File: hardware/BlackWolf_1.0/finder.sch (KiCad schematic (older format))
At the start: 13 parts, among them U4 TCA9545A, U5 VL6180X_POLOLU, U6 VL6180X_POLOLU, U7 VL6180X_POLOLU, U8 VL6180X_POLOLU

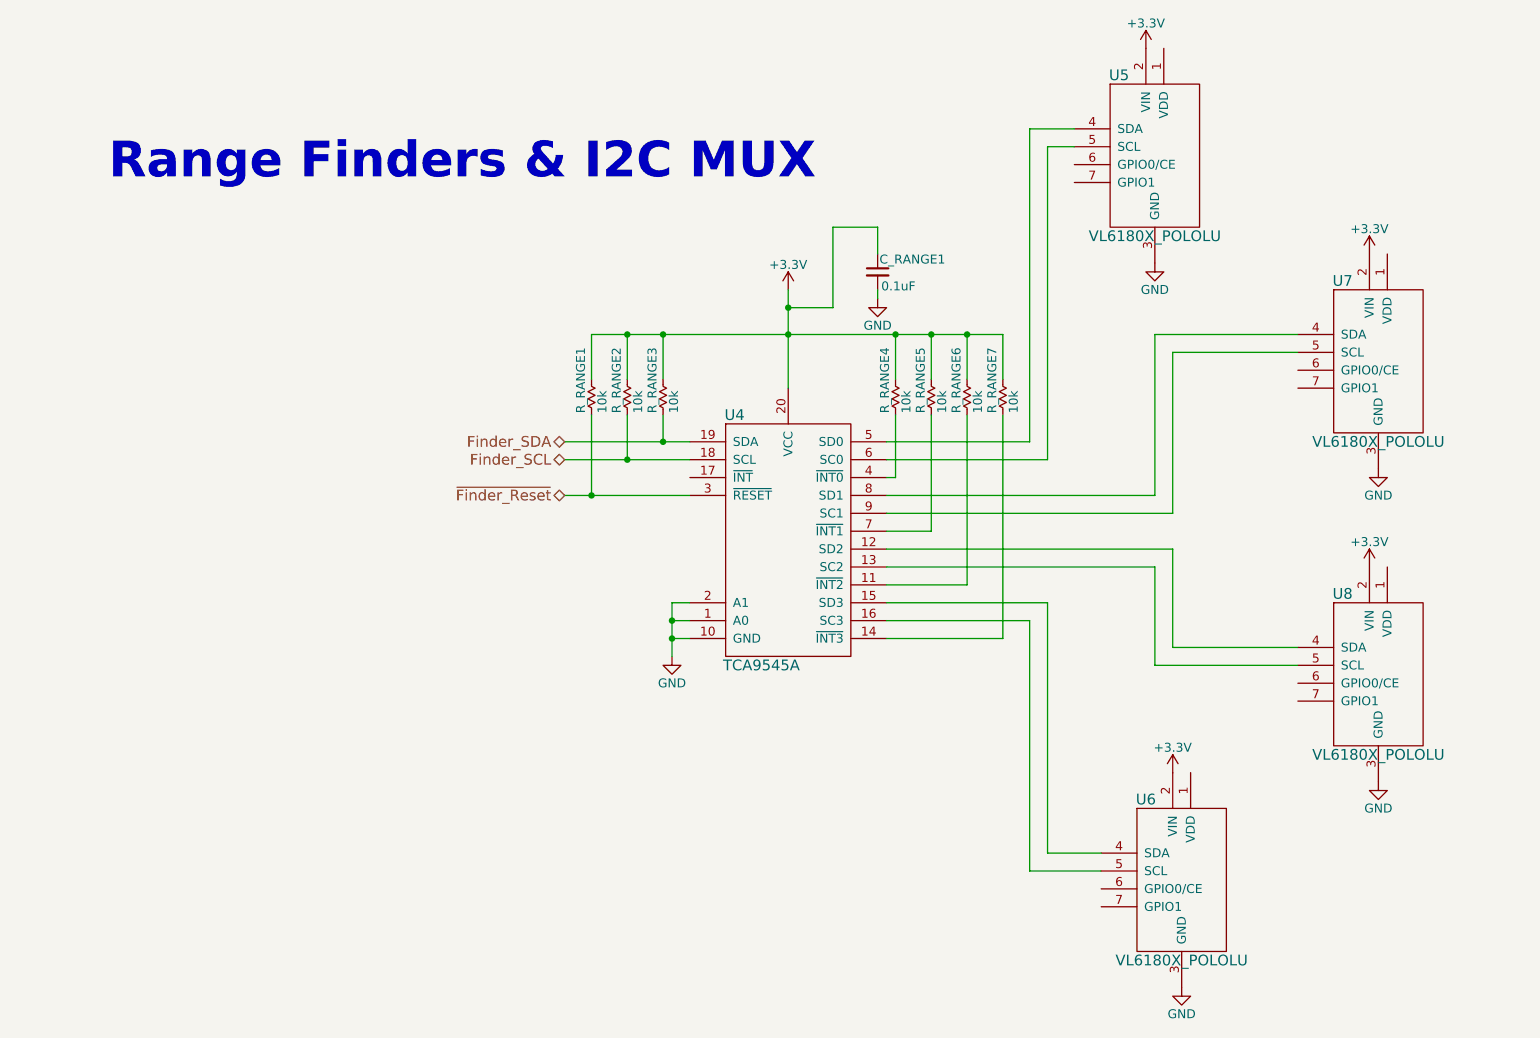
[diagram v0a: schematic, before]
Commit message: added BlackWolf hardware project - on progress!
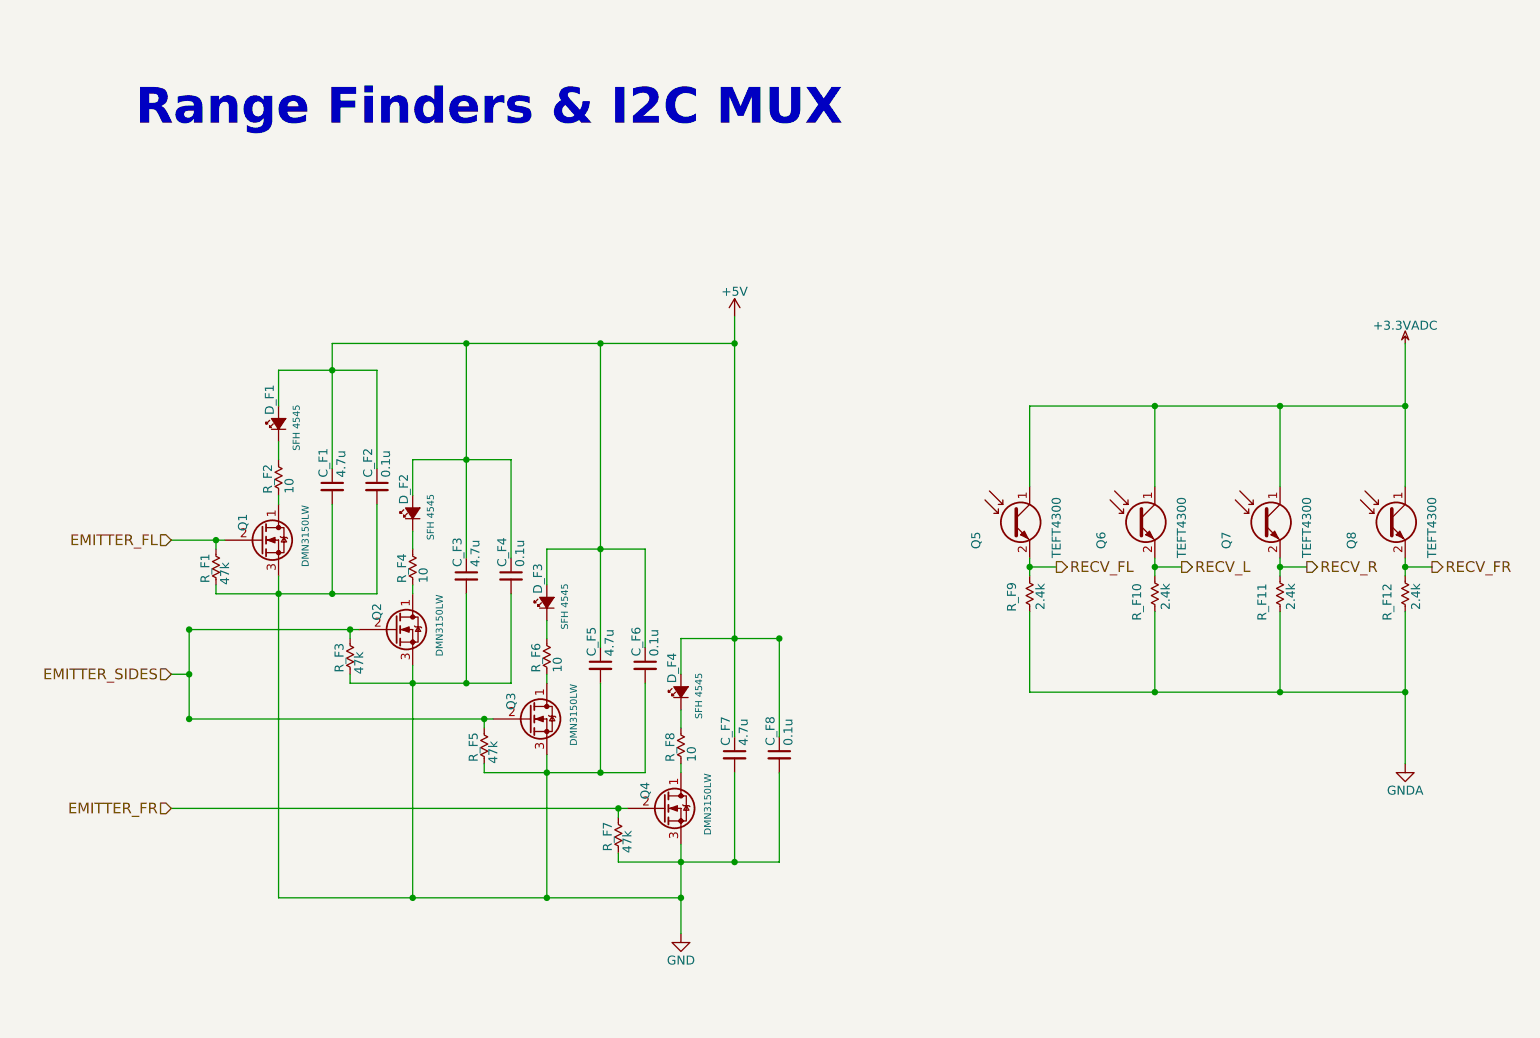
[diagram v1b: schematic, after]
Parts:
- removed C_RANGE1: 0.1uF, Capacitors_SMD:C_0603, symbol C_Small
- removed R_RANGE1, R_RANGE2, R_RANGE3, R_RANGE4, R_RANGE5, R_RANGE6, R_RANGE7: 10k, Resistors_SMD:R_0603, symbol R_Small
- removed U4: TCA9545A, Housings_SSOP:TSSOP-20_4.4x6.5mm_Pitch0.65mm, symbol TCA9545A
- removed U5, U6, U7, U8: VL6180X_POLOLU, footprints_micromouse:VL6180X_POLOLU_Pin_Header_Straight_1x07, symbol VL6180X_POLOLU
- added C_F1, C_F3, C_F5, C_F7: 4.7u, Capacitors_SMD:C_0603, symbol C_Small
- added C_F2, C_F4, C_F6, C_F8: 0.1u, Capacitors_SMD:C_0603, symbol C_Small
- added D_F1, D_F2, D_F3, D_F4: SFH 4545, Pin_Headers:Pin_Header_Straight_1x02_Pitch2.54mm, symbol Led_Small
- added Q1, Q2, Q3, Q4: DMN3150LW, TO_SOT_Packages_SMD:SOT-323_SC-70, symbol Q_NMOS_DGS
- added Q5, Q6, Q7, Q8: TEFT4300, Pin_Headers:Pin_Header_Straight_1x02_Pitch2.54mm, symbol Q_Photo_NPN
- added R_F1, R_F3, R_F5, R_F7: 47k, Resistors_SMD:R_0603, symbol R_Small
- added R_F10, R_F11, R_F12, R_F9: 2.4k, Resistors_SMD:R_0603, symbol R_Small
- added R_F2, R_F4, R_F6, R_F8: 10, Resistors_SMD:R_0603, symbol R_Small
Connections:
- net GND: now also C_F1.2, C_F2.2, C_F3.2, C_F4.2, C_F5.2, C_F6.2, C_F7.2, C_F8.2, Q1.3 (S), Q2.3 (S), Q3.3 (S), Q4.3 (S), R_F1.2, R_F3.2, R_F5.2, R_F7.2
- new net: Q1.1 (D), R_F2.2
- new net: D_F1.1 (K), R_F2.1
- new net: Q2.1 (D), R_F4.2
- new net: D_F2.1 (K), R_F4.1
- new net: Q3.1 (D), R_F6.2
- new net: D_F3.1 (K), R_F6.1
- new net: Q4.1 (D), R_F8.2
- new net: D_F4.1 (K), R_F8.1
- new net +3.3VADC: Q5.1 (C), Q6.1 (C), Q7.1 (C), Q8.1 (C)
- new net +5V: C_F1.1, C_F2.1, C_F3.1, C_F4.1, C_F5.1, C_F6.1, C_F7.1, C_F8.1, D_F1.2 (A), D_F2.2 (A), D_F3.2 (A), D_F4.2 (A)
- new net EMITTER_FL: Q1.2 (G), R_F1.1
- new net EMITTER_FR: Q4.2 (G), R_F7.1
- new net EMITTER_SIDES: Q2.2 (G), Q3.2 (G), R_F3.1, R_F5.1
- new net GNDA: R_F10.2, R_F11.2, R_F12.2, R_F9.2
- new net RECV_FL: Q5.2 (E), R_F9.1
- new net RECV_FR: Q8.2 (E), R_F12.1
- new net RECV_L: Q6.2 (E), R_F10.1
- new net RECV_R: Q7.2 (E), R_F11.1
